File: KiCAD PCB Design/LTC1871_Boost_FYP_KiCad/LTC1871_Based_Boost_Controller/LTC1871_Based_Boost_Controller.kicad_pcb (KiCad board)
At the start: 2 copper layers, 28 parts, among them Q1 IRF7811, U1 LTC1871EMS-7-PBF

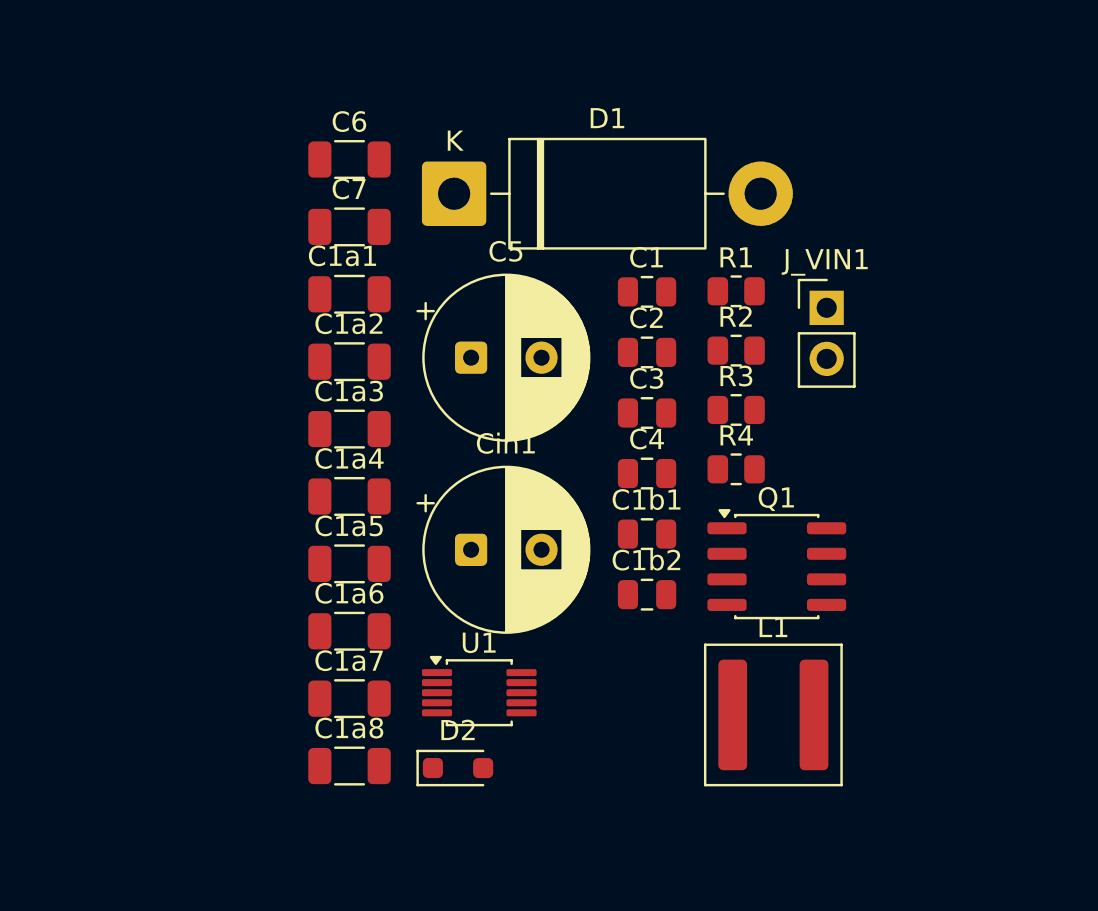
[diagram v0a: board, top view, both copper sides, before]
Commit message: Auto-sync from Fortune at 2026-04-08 16:47:45
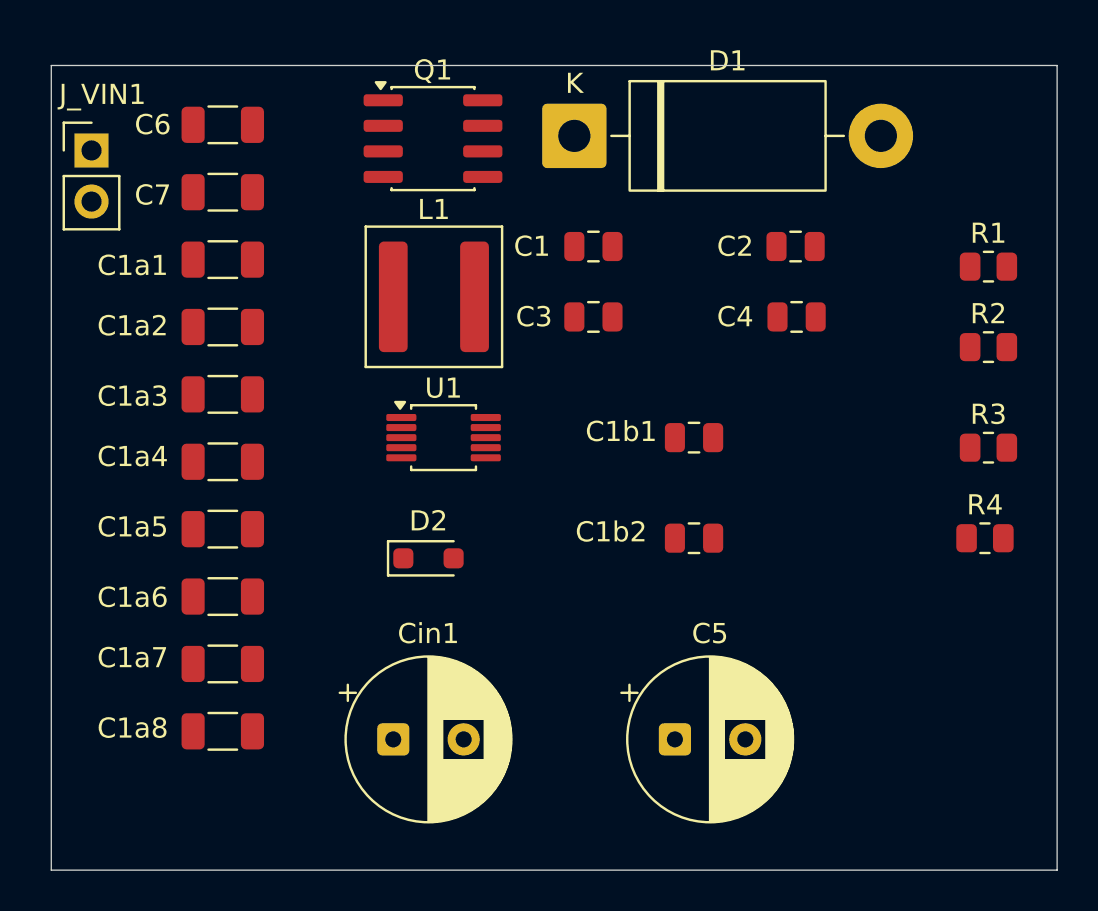
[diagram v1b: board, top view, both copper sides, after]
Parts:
- moved J_VIN1 37.4 mm to (115.5, 79.2)
- moved Q1 27.3 mm to (132.5, 78.6)
- moved L1 26.8 mm to (132.5, 86.5)
- moved C5 21.5 mm to (144.5, 108.5)
- moved R4 12.8 mm to (159.9, 98.5)
- moved U1 12.8 mm to (133.0, 93.5)
- moved R3 12.7 mm to (160.1, 94.0)
- moved R1 12.6 mm to (160.1, 85.0)
- moved R2 12.5 mm to (160.1, 89.0)
- moved C4 10.8 mm to (150.6, 87.5)
- moved D2 10.5 mm to (132.2, 99.5)
- moved Cin1 10.2 mm to (130.5, 108.5)
- moved C2 9.07 mm to (150.5, 84.0)
- moved D1 6.63 mm to (139.5, 78.5)
- moved C1a3 6.53 mm to (122.0, 91.3)
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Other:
- board outline added: 50 x 40 mm
